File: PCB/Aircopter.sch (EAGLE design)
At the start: 0 parts

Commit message: Update Schematic
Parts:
- added *1: STM32L432KCU6STM32L432KCU6_QFN32_5X5MM, Aircopter:STM32L432KCU6STM32L432KCU6_QFN32_5X5MM
- added *2: DSC6001CI1A-008.0000TDSC6001CI1A-008.0000T_VFLGA4, Aircopter:DSC6001CI1A-008.0000TDSC6001CI1A-008.0000T_VFLGA4
- added *3: TPS63001DRCRTPS63001DRCR_VSON10, Aircopter:TPS63001DRCRTPS63001DRCR_VSON10
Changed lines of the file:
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@@
 <grid distance="0.1" unitdist="inch" unit="inch" style="lines" multiple="1" display="no" altdistance="0.01" altunitdist="inch" altunit="inch"/>
 <layers>
+<layer number="1" name="Top" color="4" fill="1" visible="no" active="no"/>
+<layer number="2" name="Route2" color="1" fill="3" visible="no" active="no"/>
+<layer number="3" name="Route3" color="4" fill="3" visible="no" active="no"/>
+<layer number="4" name="Route4" color="1" fill="4" visible="no" active="no"/>
+<layer number="5" name="Route5" color="4" fill="4" visible="no" active="no"/>
+<layer number="6" name="Route6" color="1" fill="8" visible="no" active="no"/>
+<layer number="7" name="Route7" color="4" fill="8" visible="no" active="no"/>
+<layer number="8" name="Route8" color="1" fill="2" visible="no" active="no"/>
+<layer number="9" name="Route9" color="4" fill="2" visible="no" active="no"/>
+<layer number="10" name="Route10" color="1" fill="7" visible="no" active="no"/>
+<layer number="11" name="Route11" color="4" fill="7" visible="no" active="no"/>
+<layer number="12" name="Route12" color="1" fill="5" visible="no" active="no"/>
+<layer number="13" name="Route13" color="4" fill="5" visible="no" active="no"/>
+<layer number="14" name="Route14" color="1" fill="6" visible="no" active="no"/>
+<layer number="15" name="Route15" color="4" fill="6" visible="no" active="no"/>
+<layer number="16" name="Bottom" color="1" fill="1" visible="no" active="no"/>
+<layer number="17" name="Pads" color="2" fill="1" visible="no" active="no"/>
+<layer number="18" name="Vias" color="2" fill="1" visible="no" active="no"/>
+<layer number="19" name="Unrouted" color="6" fill="1" visible="no" active="no"/>
+<layer number="20" name="Dimension" color="15" fill="1" visible="no" active="no"/>
+<layer number="21" name="tPlace" color="7" fill="1" visible="no" active="no"/>
+<layer number="22" name="bPlace" color="7" fill="1" visible="no" active="no"/>
+<layer number="23" name="tOrigins" color="15" fill="1" visible="no" active="no"/>
+<layer number="24" name="bOrigins" color="15" fill="1" visible="no" active="no"/>
+<layer number="25" name="tNames" color="7" fill="1" visible="no" active="no"/>
+<layer number="26" name="bNames" color="7" fill="1" visible="no" active="no"/>
+<layer number="27" name="tValues" color="7" fill="1" visible="no" active="no"/>
+<layer number="28" name="bValues" color="7" fill="1" visible="no" active="no"/>
+<layer number="29" name="tStop" color="7" fill="3" visible="no" active="no"/>
+<layer number="30" name="bStop" color="7" fill="6" visible="no" active="no"/>
+<layer number="31" name="tCream" color="7" fill="4" visible="no" active="no"/>
+<layer number="32" name="bCream" color="7" fill="5" visible="no" active="no"/>
+<layer number="33" name="tFinish" color="6" fill="3" visible="no" active="no"/>
+<layer number="34" name="bFinish" color="6" fill="6" visible="no" active="no"/>
+<layer number="35" name="tGlue" color="7" fill="4" visible="no" active="no"/>
+<layer number="36" name="bGlue" color="7" fill="5" visible="no" active="no"/>
+<layer number="37" name="tTest" color="7" fill="1" visible="no" active="no"/>
+<layer number="38" name="bTest" color="7" fill="1" visible="no" active="no"/>
+<layer number="39" name="tKeepout" color="4" fill="11" visible="no" active="no"/>
+<layer number="40" name="bKeepout" color="1" fill="11" visible="no" active="no"/>
+<layer number="41" name="tRestrict" color="4" fill="10" visible="no" active="no"/>
+<layer number="42" name="bRestrict" color="1" fill="10" visible="no" active="no"/>
+<layer number="43" name="vRestrict" color="2" fill="10" visible="no" active="no"/>
+<layer number="44" name="Drills" color="7" fill="1" visible="no" active="no"/>
+<layer number="45" name="Holes" color="7" fill="1" visible="no" active="no"/>
+<layer number="46" name="Milling" color="3" fill="1" visible="no" active="no"/>
+<layer number="47" name="Measures" color="7" fill="1" visible="no" active="no"/>
+<layer number="48" name="Document" color="7" fill="1" visible="no" active="no"/>
+<layer number="49" name="Reference" color="7" fill="1" visible="no" active="no"/>
+<layer number="51" name="tDocu" color="7" fill="1" visible="no" active="no"/>
+<layer number="52" name="bDocu" color="7" fill="1" visible="no" active="no"/>
 <layer number="88" name="SimResults" color="9" fill="1" visible="yes" active="yes"/>
 <layer number="89" name="SimProbes" color="9" fill="1" visible="yes" active="yes"/>
@@
 </classes>
 <parts>
+<part name="*1" library="Aircopter" library_urn="urn:adsk.eagle:library:7112503" deviceset="STM32L432KCU6" device="STM32L432KCU6_QFN32_5X5MM" package3d_urn="urn:adsk.eagle:package:7112519/1"/>
+<part name="*2" library="Aircopter" library_urn="urn:adsk.eagle:library:7112503" deviceset="DSC6001CI1A-008.0000T" device="DSC6001CI1A-008.0000T_VFLGA4" package3d_urn="urn:adsk.eagle:package:7112517/1"/>
+<part name="*3" library="Aircopter" library_urn="urn:adsk.eagle:library:7112503" deviceset="TPS63001DRCR" device="TPS63001DRCR_VSON10" package3d_urn="urn:adsk.eagle:package:7112518/1"/>
 </parts>
 <sheets>
@@
 </plain>
 <instances>
+<instance part="*1" gate="A" x="20.32" y="55.88" smashed="yes">
+<attribute name="NAME" x="21.59" y="57.15" size="1.27" layer="95"/>
+<attribute name="VALUE" x="19.05" y="3.81" size="1.27" layer="96"/>
+</instance>
+<instance part="*2" gate="A" x="104.14" y="48.26" smashed="yes">
+<attribute name="NAME" x="102.87" y="49.53" size="1.27" layer="95"/>
+<attribute name="VALUE" x="87.63" y="41.91" size="1.27" layer="96"/>
+</instance>
+<instance part="*3" gate="A" x="99.06" y="27.94" smashed="yes">
+<attribute name="NAME" x="97.79" y="29.21" size="1.27" layer="95"/>
+<attribute name="VALUE" x="90.17" y="11.43" size="1.27" layer="96"/>
+</instance>
 </instances>
 <busses>
@@
 </schematic>
 </drawing>
+<compatibility>
+<note version="8.2" severity="warning">
+Since Version 8.2, EAGLE supports online libraries. The ids
+of those online libraries will not be understood (or retained)
+with this version.
+</note>
+<note version="8.3" severity="warning">
+Since Version 8.3, EAGLE supports URNs for individual library
+assets (packages, symbols, and devices). The URNs of those assets
+will not be understood (or retained) with this version.
+</note>
+<note version="8.3" severity="warning">
+Since Version 8.3, EAGLE supports the association of 3D packages
+with devices in libraries, schematics, and board files. Those 3D
+packages will not be understood (or retained) with this version.
+</note>
+</compatibility>
 </eagle>

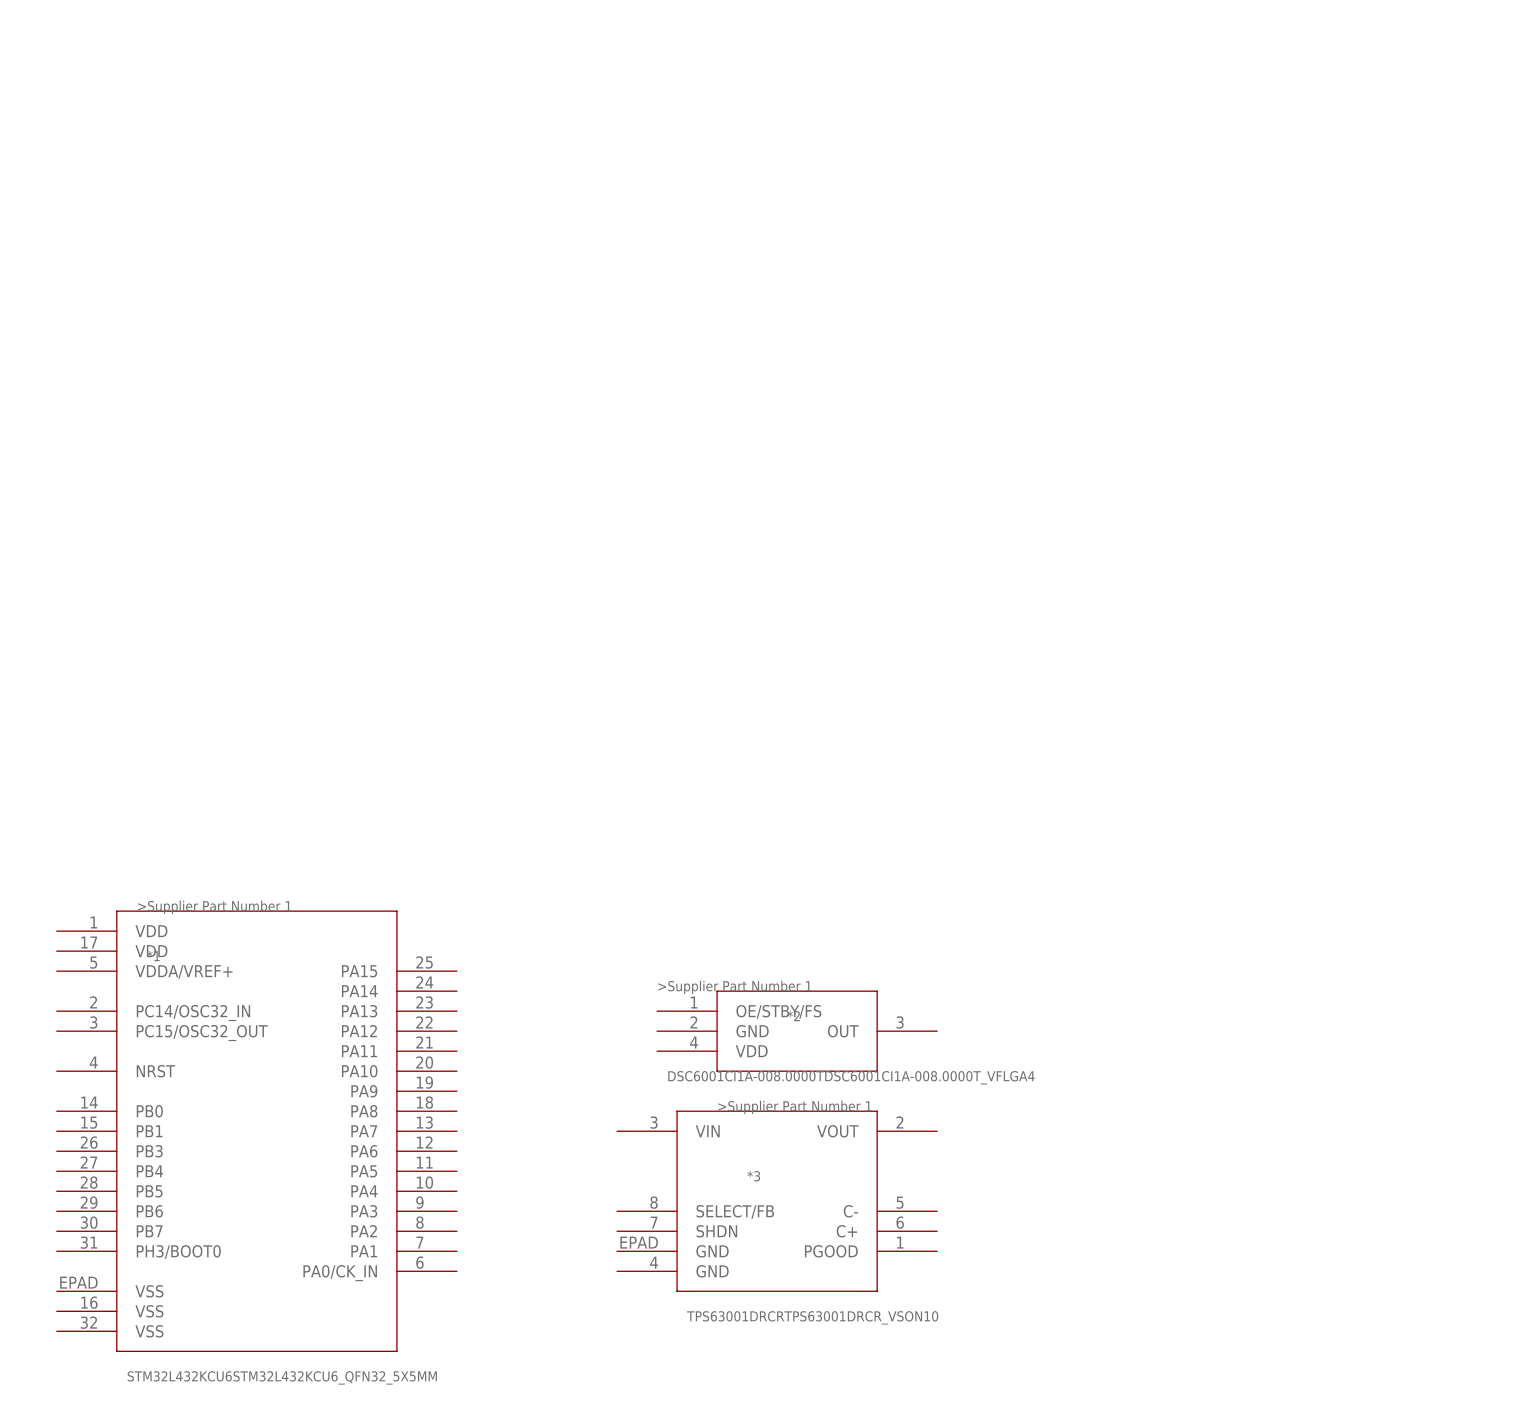
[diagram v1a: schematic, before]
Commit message: Update Sch
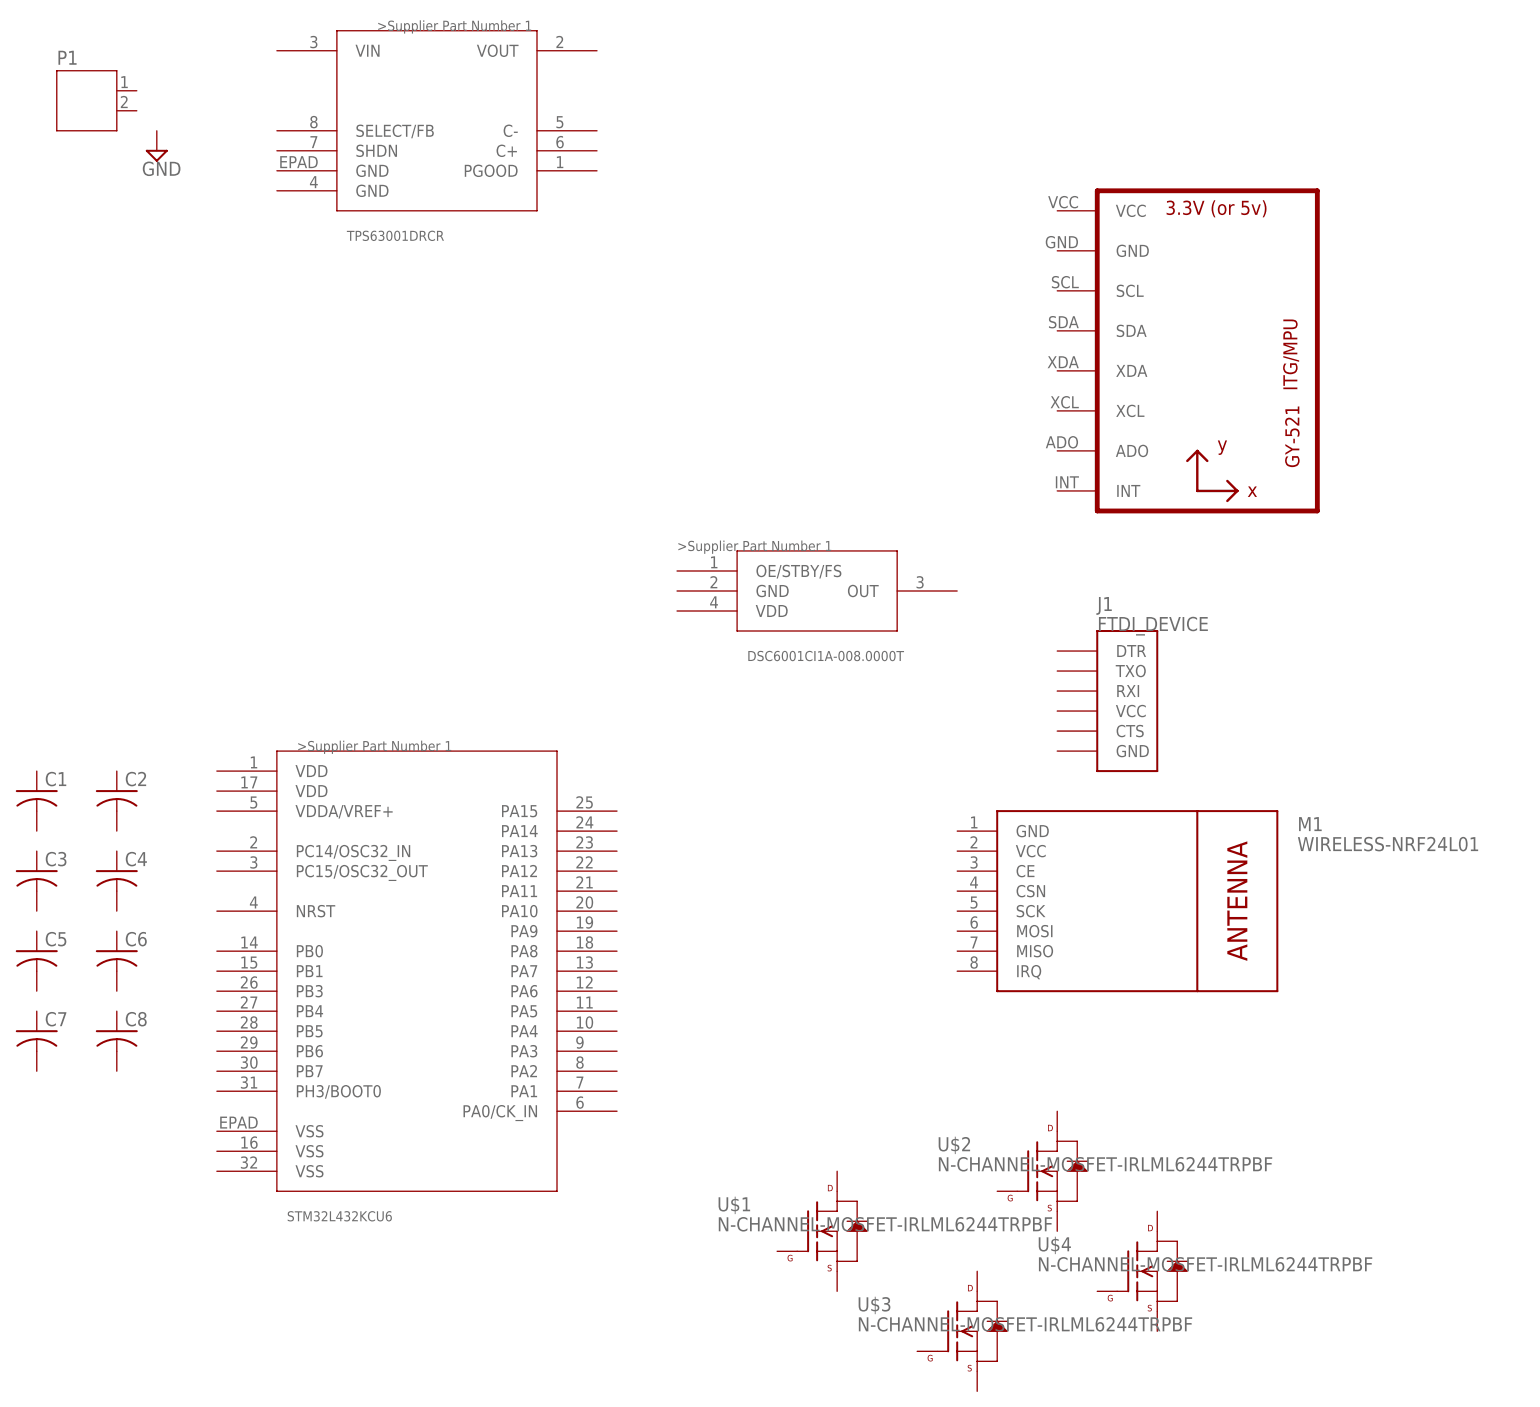
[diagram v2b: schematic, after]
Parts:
- added C1, C2, C3, C4, C5, C6, C7, C8: (no value), rcl:C-USC0603K
- added J1: FTDI_DEVICE, AP_quad:FTDI_DEVICE
- added M1: WIRELESS-NRF24L01, AP_quad:WIRELESS-NRF24L01
- added P1: (no value), jst-ph:JST-PH2
- added U$1, U$2, U$3, U$4: N-CHANNEL-MOSFET-IRLML6244TRPBF, AP_quad:N-CHANNEL-MOSFET-IRLML6244TRPBF
- added U1: GY-521MPU6050, AP_quad:GY-521MPU6050
- *1: value STM32L432KCU6STM32L432KCU6_QFN32_5X5MM -> STM32L432KCU6
- *2: value DSC6001CI1A-008.0000TDSC6001CI1A-008.0000T_VFLGA4 -> DSC6001CI1A-008.0000T
- *3: value TPS63001DRCRTPS63001DRCR_VSON10 -> TPS63001DRCR
